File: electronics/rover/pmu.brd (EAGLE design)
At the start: 55.2 x 38.4 mm, 41 parts, among them U1 L5973D, U2 L5973D, U3 L5973D

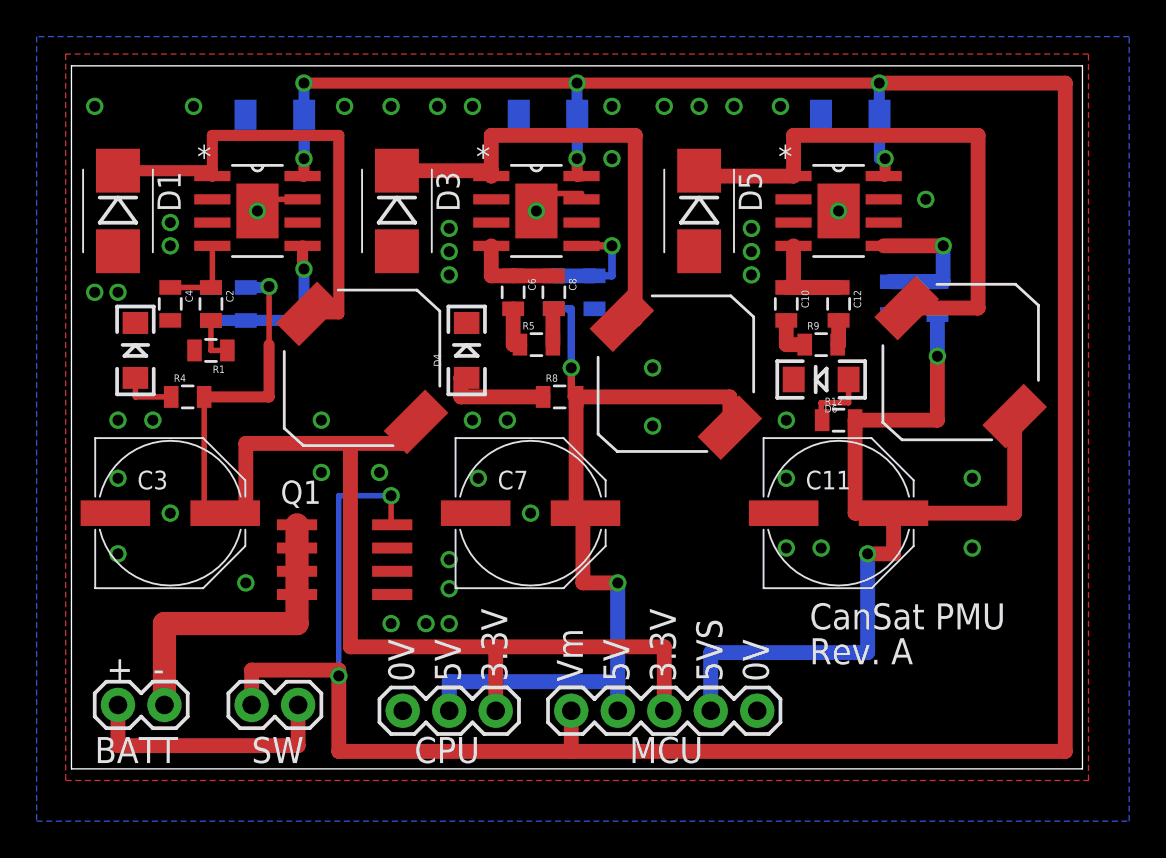
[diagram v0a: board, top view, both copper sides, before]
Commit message: Added new electronic designs
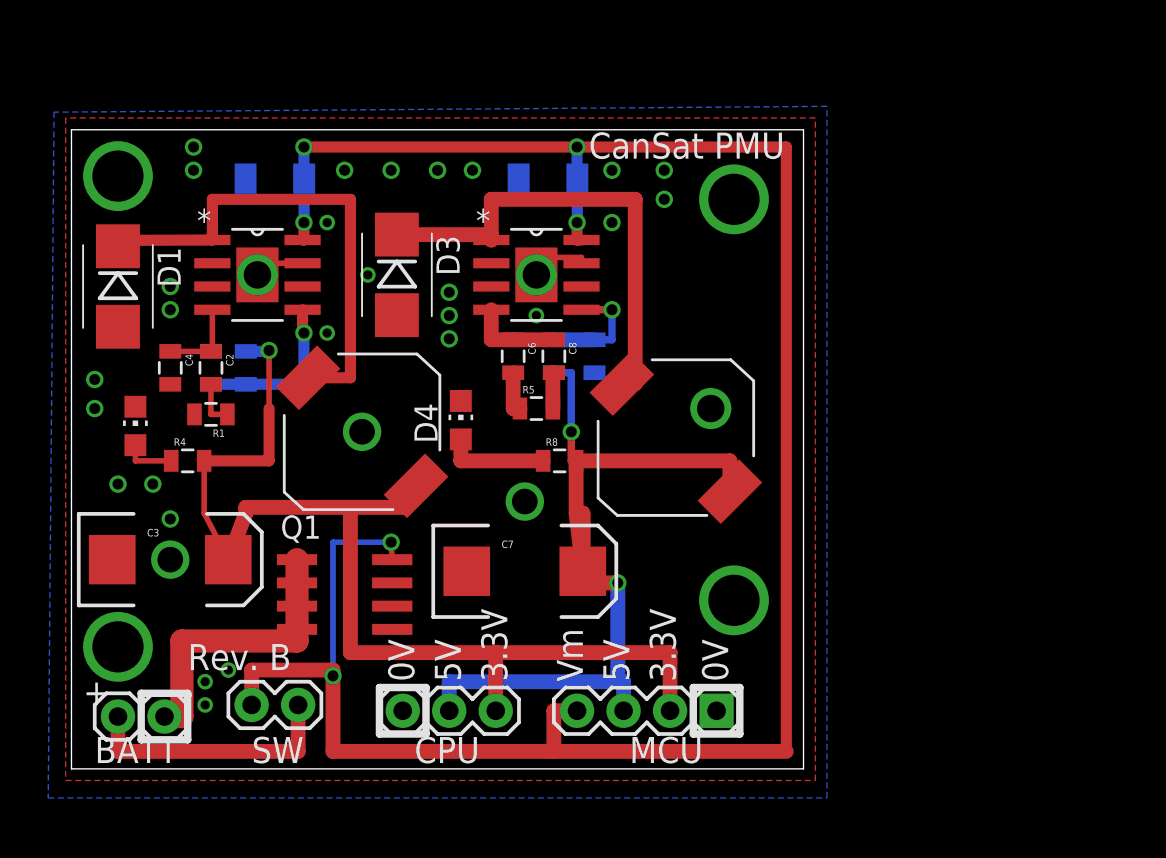
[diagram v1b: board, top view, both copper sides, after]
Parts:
- removed C10: 22n, SparkFun-Passives:0805
- removed C11: 330u, rcl:PANASONIC_E
- removed C12: 220p, SparkFun-Passives:0805
- removed C9: 10u, SparkFun-Passives:1210
- removed D5: (no value), SparkFun-DiscreteSemi:SMB-DIODE
- removed D6: GREEN, SparkFun-LED:LED-1206
- removed L3: 15uH, Panasonic-ELL:IND_ELL8TP
- removed MCU_PWR: (no value), SparkFun-Connectors:1X05
- removed R10: 8.2k, SparkFun-Passives:0805
- removed R11: 2.7k, SparkFun-Passives:0805
- removed R12: 330, SparkFun-Passives:0805
- removed R9: 4k7, SparkFun-Passives:0805
- removed U3: L5973D, L5973D:SOP127P600X170-9N
- added JP1: (no value), SparkFun-Connectors:1X04
- C3, C7: device rcl:PANASONIC_E -> SparkFun-Passives:EIA7343
- D2, D4: device SparkFun-LED:LED-1206 -> led:CHIP-LED0805
- moved D1 4.13 mm to (2.54, 26.4)
- moved D2 4.13 mm to (3.49, 18.7), turned to 0 degrees
- moved D4 3.82 mm to (21.3, 19.1), turned to 0 degrees
- moved C1 3.49 mm to (11.1, 32.1)
- moved C2 3.49 mm to (7.62, 21.9)
- moved C4 3.49 mm to (5.40, 21.9)
- moved C5 3.49 mm to (26.0, 32.1)
- moved C6 3.49 mm to (24.1, 22.5)
- moved C8 3.49 mm to (26.4, 22.5)
- moved D3 3.49 mm to (17.8, 27.0)
- moved L1 3.49 mm to (15.9, 18.4)
- moved L2 3.49 mm to (33.0, 18.1)
- moved R1 3.49 mm to (7.62, 19.4)
- moved R2 3.49 mm to (9.53, 21.9)
- moved R3 3.49 mm to (7.62, 21.9)
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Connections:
- removed net 5VS: C11.+, L3.1, MCU_PWR.2, R10.2, R12.2
- removed net N$13: C10.2, R9.1
- removed net N$14: D5.C, L3.2, U3.1
- removed net N$15: R10.1, R11.2, U3.5
- removed net N$16: D6.A, R12.1
- removed net N$19: U3.6
- removed net N$7: C10.1, C12.1, U3.4
- net 3.3V: now also C3.A, JP1.2; no longer C3.+, MCU_PWR.3
- net 5V: now also C7.A, JP1.3; no longer C7.+, MCU_PWR.4
- net GND: now also C3.C, C7.C, JP1.1; no longer C11.-, C12.2, C3.-, C7.-, C9.2, D5.A, D6.C, MCU_PWR.1, R11.1, R9.2, U3.3, U3.7, U3.9
- net V_BATT: now also JP1.4; no longer C9.1, MCU_PWR.5, U3.8
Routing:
- net 5VS: track 50.1 -> 0.00 mm, vias 2 -> 0
- net V_BATT: track 161.5 -> 120.4 mm, vias 8 -> 6
- net N$14: track 31.1 -> 0.00 mm
- net N$15: track 10.6 -> 0.00 mm, vias 1 -> 0
- net N$7: track 7.60 -> 0.00 mm
- net 3.3V: track 68.6 -> 61.4 mm
- net N$16: track 3.77 -> 0.00 mm
- net GND: track 13.4 -> 10.4 mm, vias 52 -> 37
- net 5V: track 46.6 -> 49.2 mm
- net N$13: track 2.33 -> 0.00 mm
- net N$3: track 26.0 -> 27.6 mm
- net N$4: track 17.1 -> 15.8 mm
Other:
- board size 55.2 x 38.4 mm -> 40 x 34.9 mm
- board text added: "CS13-PMU-B1"
- board text added: "Rev. B"
- board text removed: "5VS"
- board text removed: "CS13-PMU-A1"
- board text removed: "Rev. A"
